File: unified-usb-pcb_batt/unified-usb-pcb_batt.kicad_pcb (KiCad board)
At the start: 2 copper layers, 34 x 29.2 mm, 34 parts, among them J1 QI, J2 USB_C_Receptacle_USB2.0, J3 USB_Out, J4 BATT, J5 THERM, SW1 SW_SPDT, U1 SRV05-4, U2 DW01A, U3 TP4056, U4 FS8205

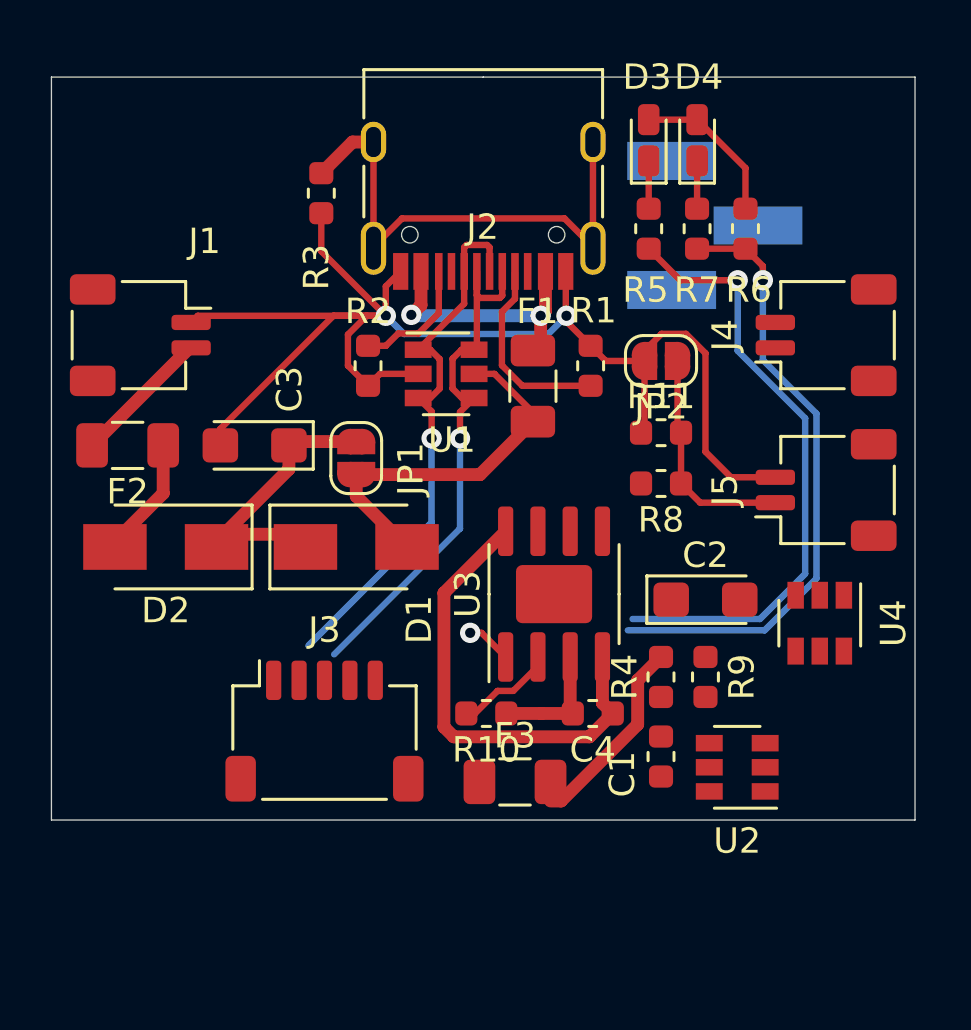
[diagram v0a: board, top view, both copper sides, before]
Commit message: finished pcb
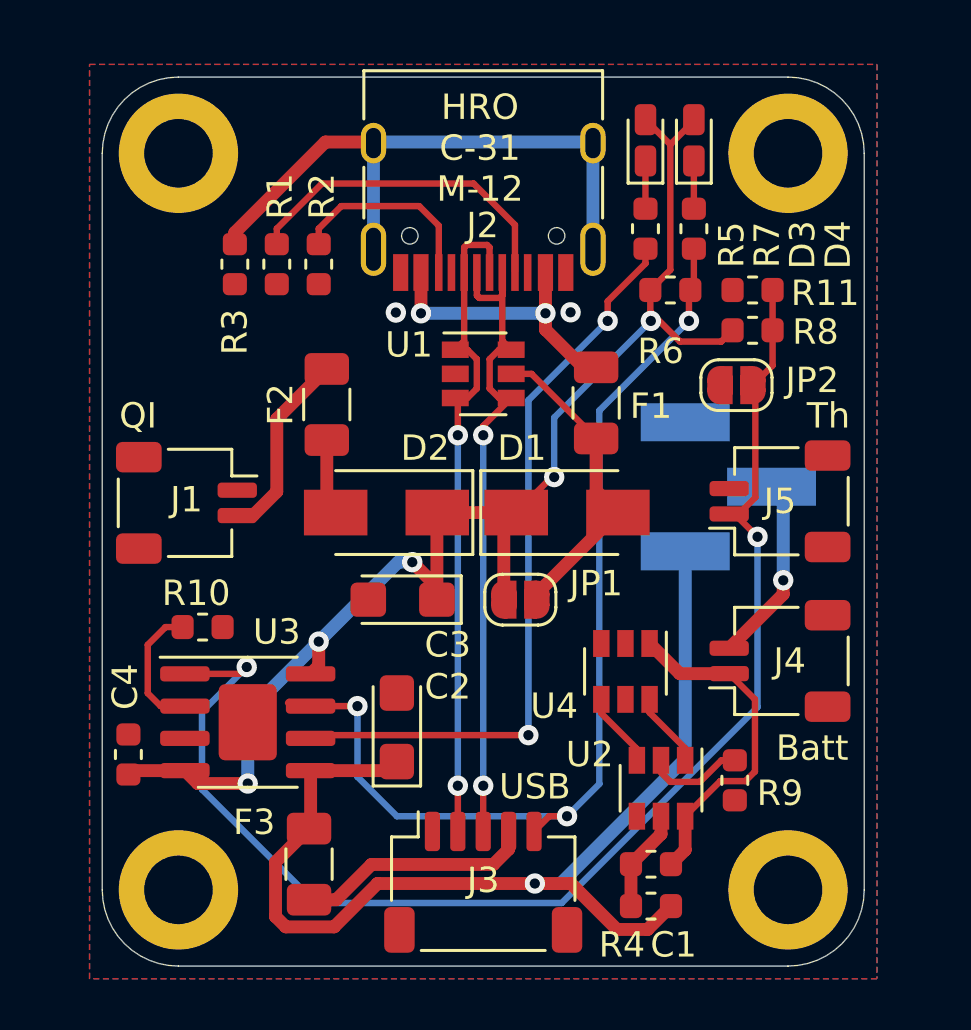
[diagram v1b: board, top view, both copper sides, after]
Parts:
- added H1: MountingHole_Pad, MountingHole:MountingHole_2.7mm_M2.5_DIN965_Pad, F.Cu at (18.8, 21.3)
- added H2: MountingHole_Pad, MountingHole:MountingHole_2.7mm_M2.5_DIN965_Pad, F.Cu at (42.8, 21.3)
- added H3: MountingHole_Pad, MountingHole:MountingHole_2.7mm_M2.5_DIN965_Pad, F.Cu at (18.8, 50.3)
- added H4: MountingHole_Pad, MountingHole:MountingHole_2.7mm_M2.5_DIN965_Pad, F.Cu at (42.8, 50.3)
- J2: value USB_C_Receptacle_USB2.0 -> HRO C-31-M-12
- moved C4 18.4 mm to (16.8, 45.0), turned to 90 degrees
- moved C2 13.1 mm to (27.4, 43.9), turned to 90 degrees
- moved U3 13.1 mm to (21.5, 43.7), turned to 0 degrees
- moved R1 13.0 mm to (22.6, 25.7), turned to 90 degrees
- moved J4 13.0 mm to (42.4, 41.3)
- moved R10 11.7 mm to (19.7, 39.9)
- moved SW1 10.3 mm to (40.4, 34.4)
- moved R4 9.03 mm to (37.4, 50.9), turned to 0 degrees
- moved D2 8.80 mm to (26.9, 35.4)
- moved F3 8.73 mm to (23.9, 49.3), turned to 90 degrees
- moved J3 8.63 mm to (30.8, 50.0)
- moved JP1 8.53 mm to (32.2, 38.9), turned to 0 degrees
- moved C3 8.42 mm to (27.6, 38.9)
- moved D1 8.41 mm to (34.1, 35.4)
- moved F2 8.00 mm to (24.6, 31.2), turned to 90 degrees
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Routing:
- net GNDPWR: track 61.0 -> 0.57 mm
- net Net-(J5-Pad1): track 10.7 -> 52.7 mm, vias 1 -> 2
- net VOUT: track 7.72 -> 43.9 mm, vias 0 -> 1
- net +5V: track 35.7 -> 53.9 mm, vias 0 -> 5
- net chgsense: track 24.3 -> 39.5 mm, vias 1 -> 3
- net Net-(C1-Pad2): track 0.00 -> 13.5 mm
- net Net-(F3-Pad1): track 0.00 -> 9.38 mm
- net Net-(J4-Pad2): track 0.00 -> 7.43 mm, vias 0 -> 1
- net Net-(J2-PadA5): track 7.74 -> 13.2 mm
- net Net-(R5-Pad1): track 24.2 -> 29.7 mm, vias 1 -> 2
- net USB_D-: track 21.6 -> 26.9 mm, vias 1 -> 2
- net USB_D+: track 21.9 -> 26.5 mm, vias 1 -> 2
- net Net-(C1-Pad1): track 0.00 -> 4.03 mm
- net Net-(R9-Pad2): track 0.00 -> 3.89 mm
- net Net-(J2-PadS1): track 20.6 -> 24.4 mm
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- added copper zone on B.Cu, net GNDPWR
- added copper zone on F.Cu, net GNDPWR
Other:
- board size 34 x 29.2 mm -> 30 x 35 mm
- board text added: "Batt"
- board text added: "HRO C-31 M-12"
- board text added: "QI"
- board text added: "Th"
- board text added: "USB"
